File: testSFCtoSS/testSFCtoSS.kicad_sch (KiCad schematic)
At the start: 13 parts, among them J1 SFC Controler, J2 SegaSaturn Controler, U1 4024, U2 NE555D, U4 4011, U5 HEF4094B, U6 HEF4094B, U7 74LS153, U8 74LS153, U9 4069

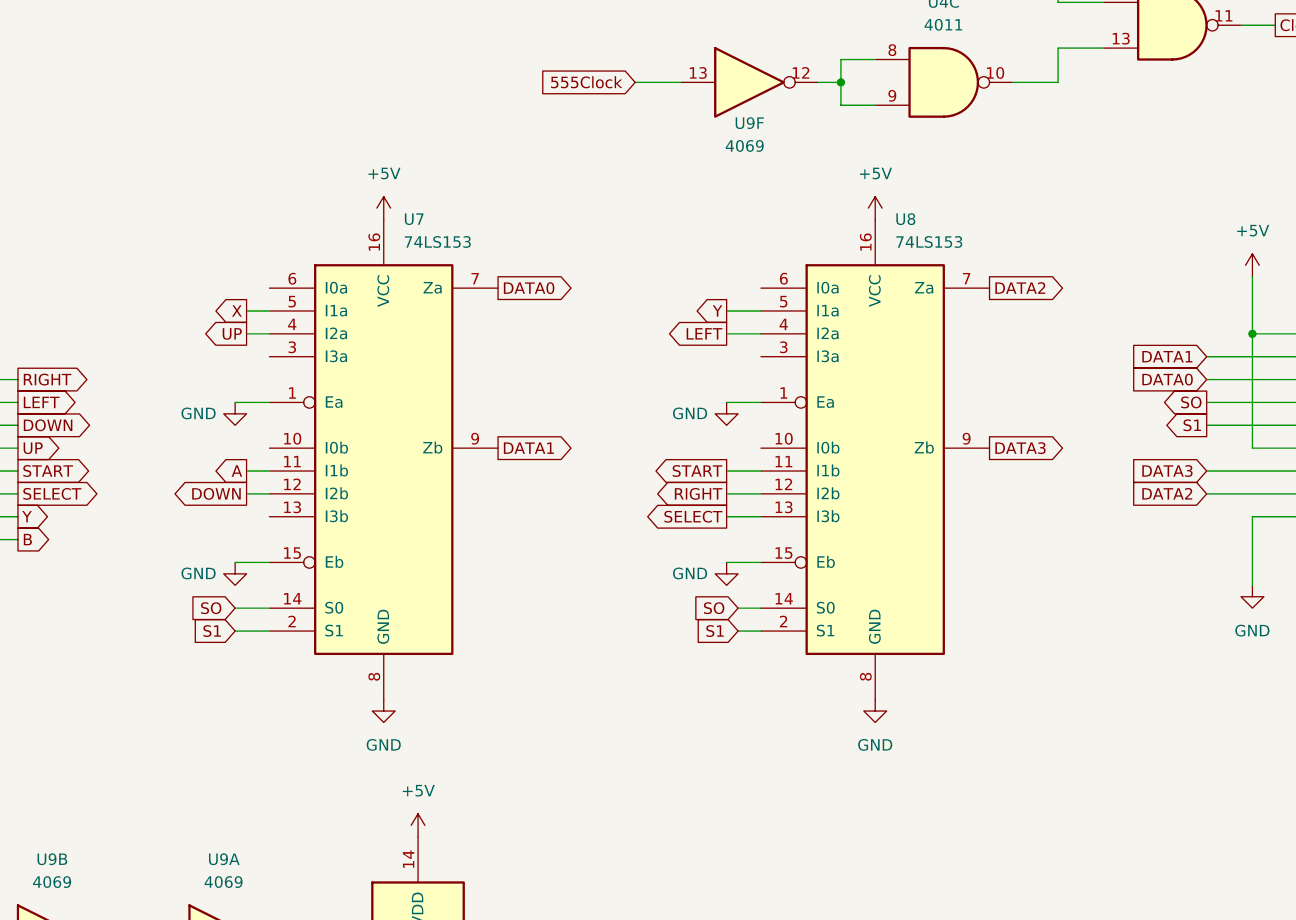
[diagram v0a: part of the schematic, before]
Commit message: update
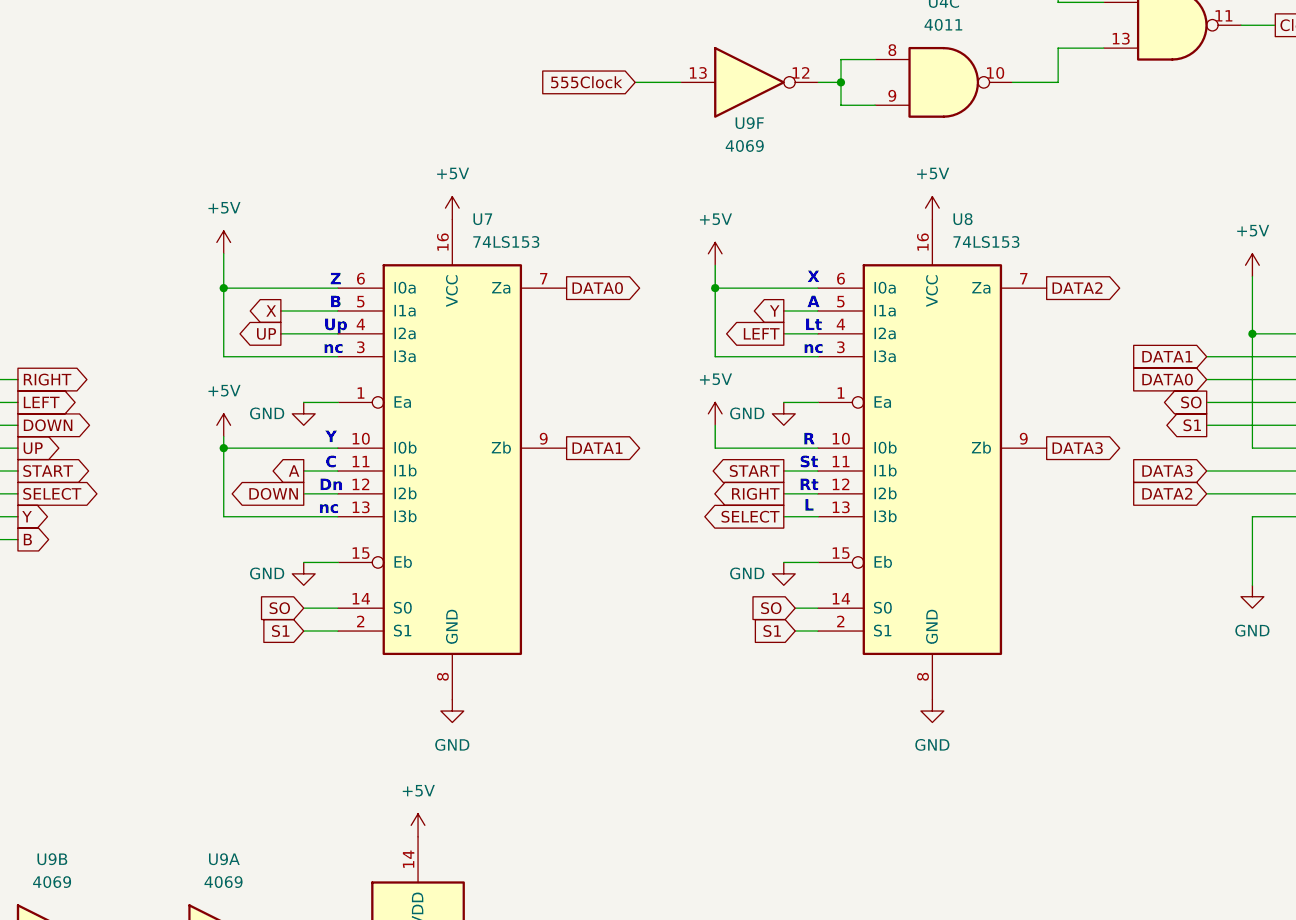
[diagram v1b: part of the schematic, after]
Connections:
- net +5V: now also U7.10 (I0b), U7.13 (I3b), U7.3 (I3a), U7.6 (I0a), U8.10 (I0b), U8.3 (I3a), U8.6 (I0a)
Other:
- note added: "A"
- note added: "B"
- note added: "C"
- note added: "Dn"
- note added: "L"
- note added: "Lt"
- note added: "R"
- note added: "Rt"
- note added: "St"
- note added: "Up"
- note added: "X"
- note added: "Y"
- note added: "Z"
- note added: "nc"
- moved on the sheet: U7, U8
